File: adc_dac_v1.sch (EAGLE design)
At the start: 24 parts, among them IC2 LT6220, IC4 LT6220, U2 DAC8832IRGYR, U4 OPA353NA/3K, U7 DAC8832IRGYR, U8 OPA353NA/3K

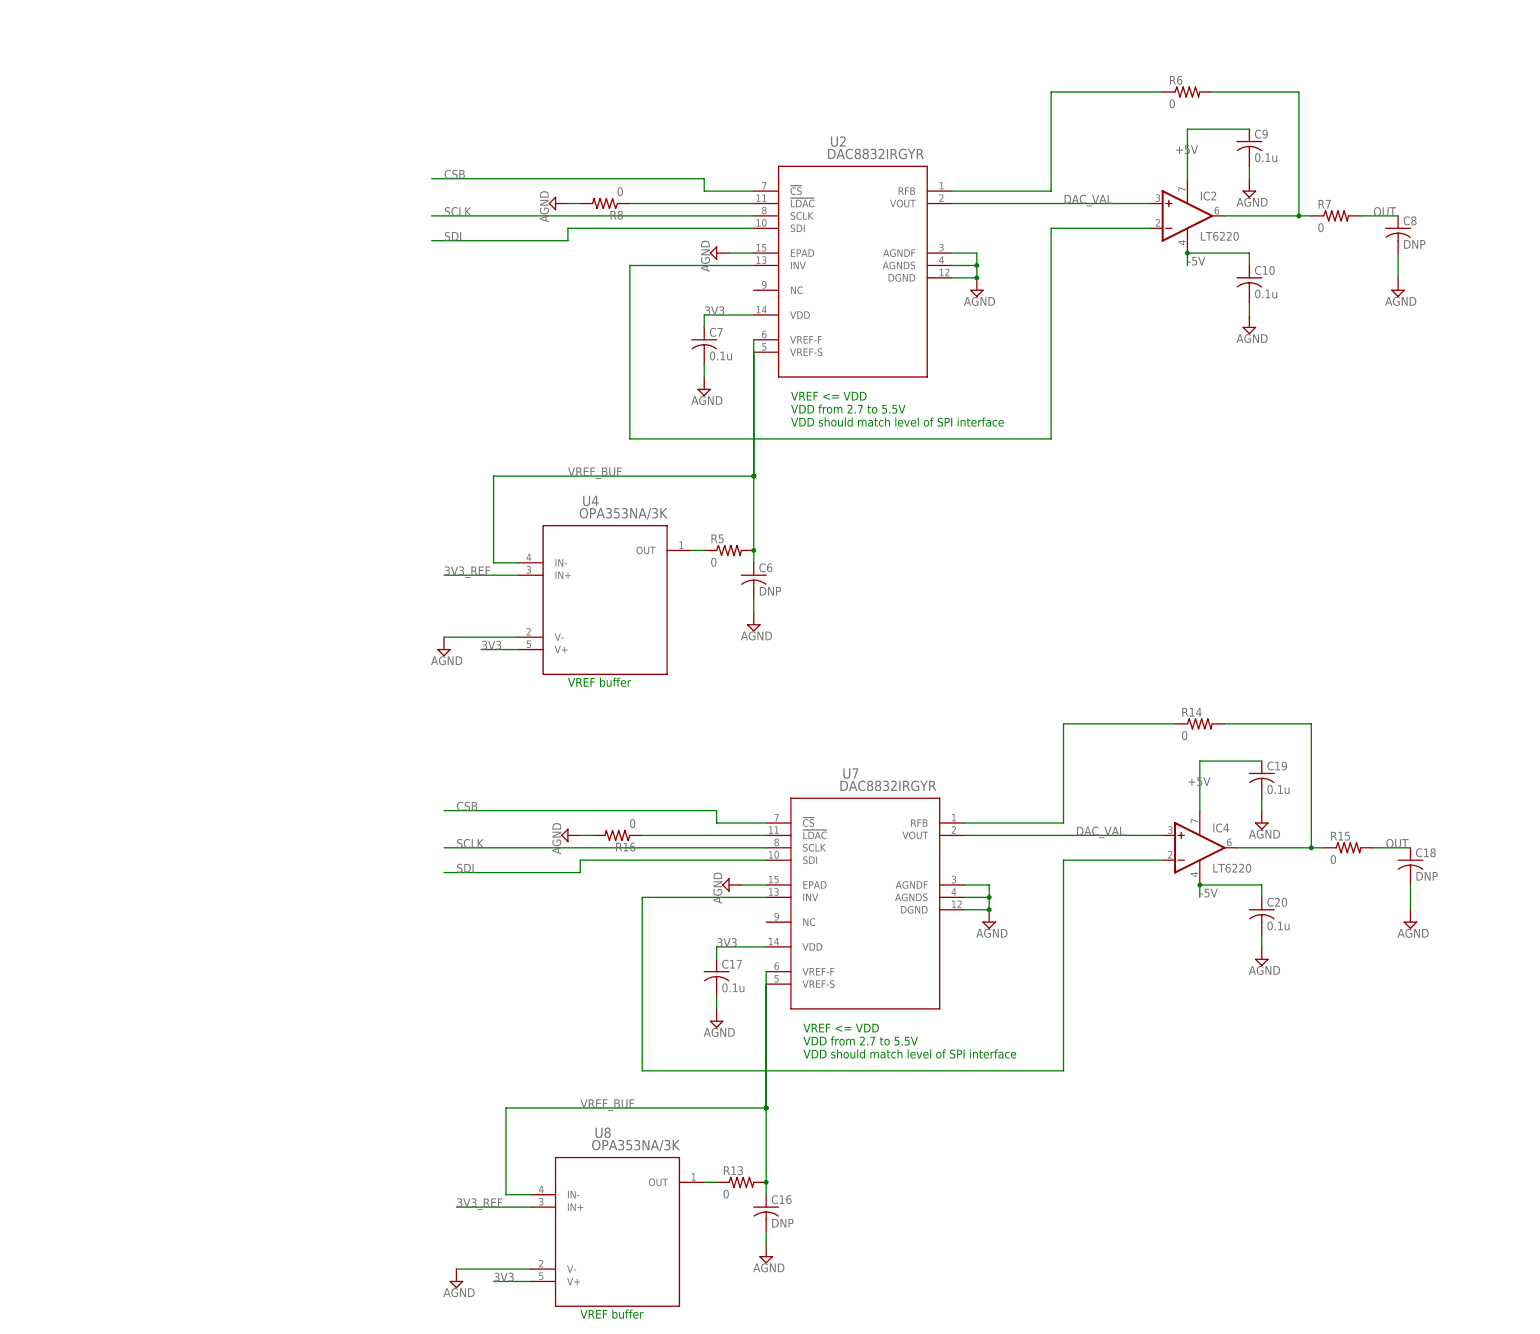
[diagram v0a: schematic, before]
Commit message: updates to DAC design
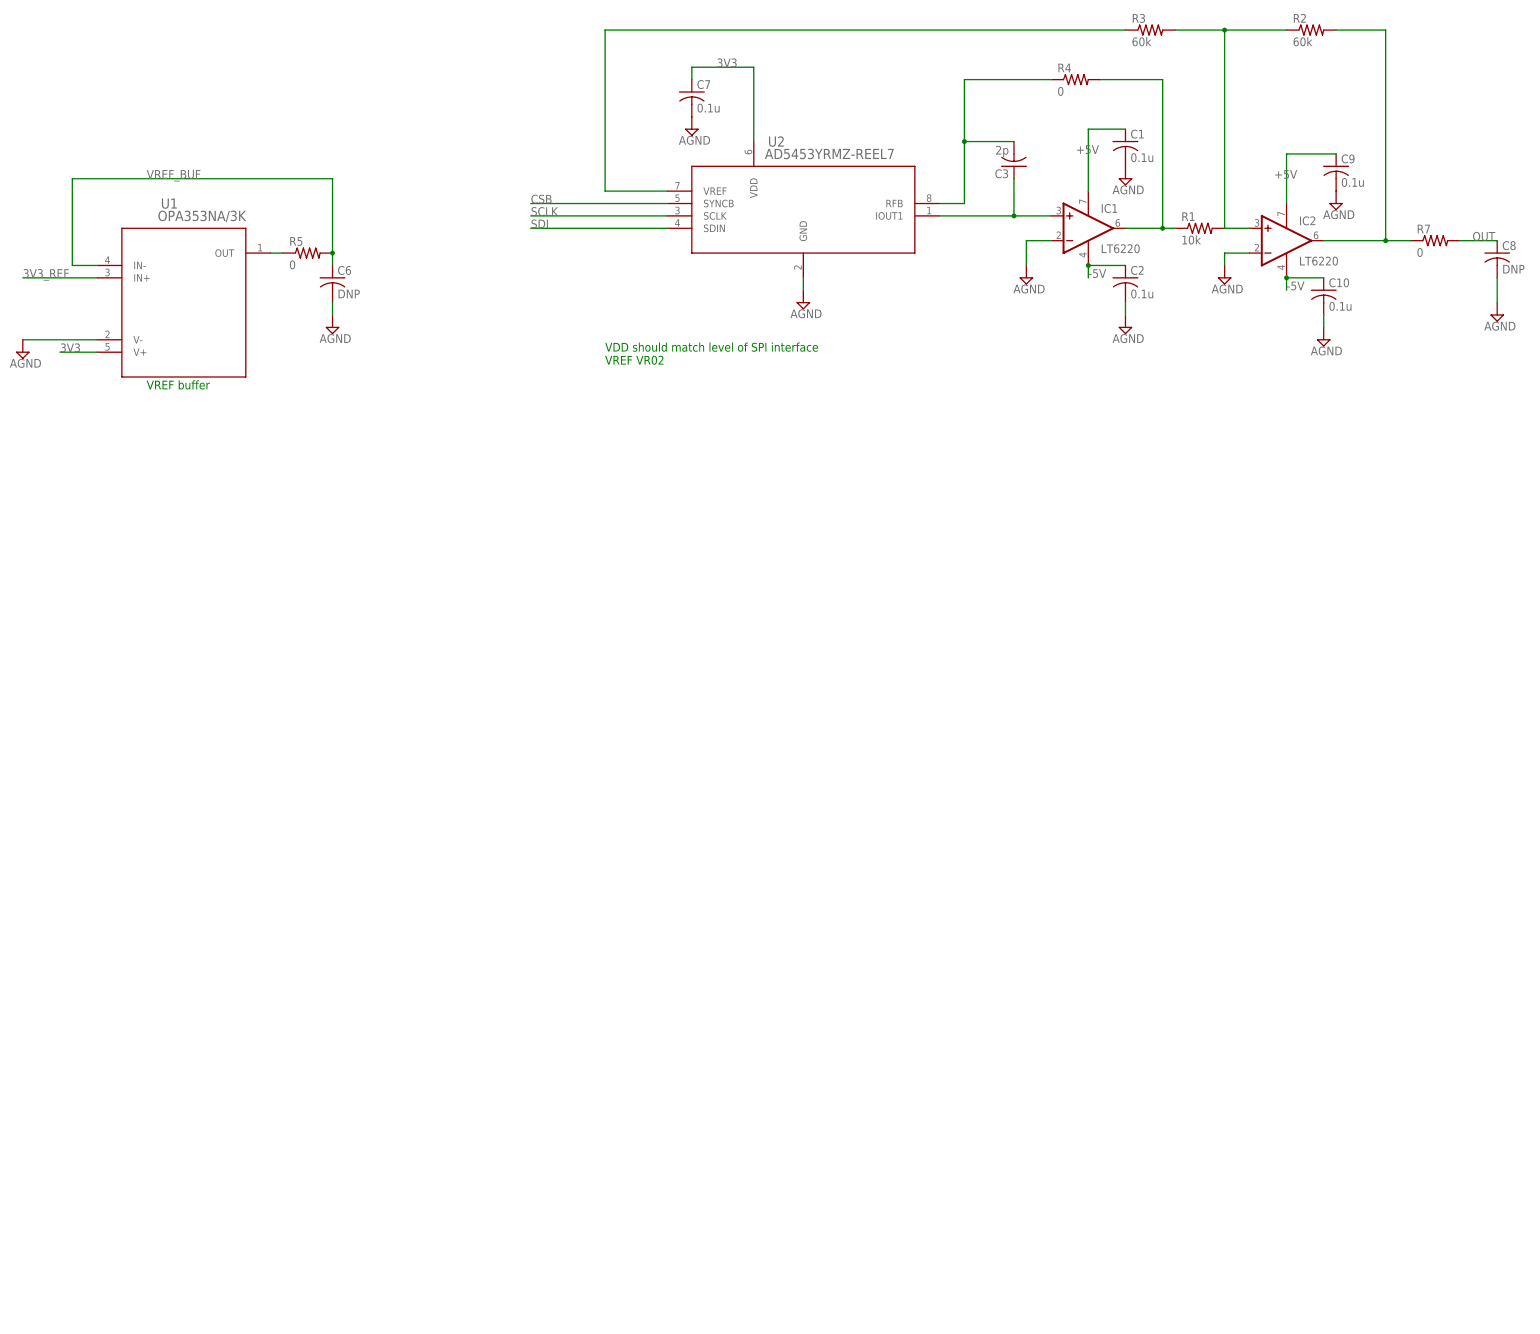
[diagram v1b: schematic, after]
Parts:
- removed C16, C18: DNP, rcl:C-USC0603
- removed C17, C19, C20: 0.1u, rcl:C-USC0603
- removed IC4: LT6220, linear:MCP601SN
- removed R13, R14, R15, R16, R6, R8: 0, rcl:R-US_R0603
- removed U4, U8: OPA353NA/3K, AD7960:OPA353NA/3K
- removed U7: DAC8832IRGYR, AD7960:DAC8832IRGYR
- added C1, C2: 0.1u, rcl:C-USC0603
- added C3: 2p, rcl:C-USC0603
- added IC1: LT6220, linear:MCP601SN
- added R1: 10k, rcl:R-US_R0603
- added R2, R3: 60k, rcl:R-US_R0603
- added R4: 0, rcl:R-US_R0603
- added U1: OPA353NA/3K, open_covg:OPA353NA/3K
- U2: value DAC8832IRGYR -> AD5453YRMZ-REEL7; device AD7960:DAC8832IRGYR -> open_covg:AD5453YRMZ-REEL7
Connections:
- removed net N$15: R14.1, U7.RFB
- removed net N$16: R16.1, U7.!LDAC
- removed net N$8: R8.1, U2.!LDAC
- new net CLK+: R2.1, U1.CLK+
- new net CLK-: R2.2, U1.CLK-
- new net CNV+: U1.CNV+
- new net CNV-: U1.CNV-
- new net D+: U1.D+
- new net D-: U1.D-
- new net DCO+: U1.DCO+
- new net DCO-: U1.DCO-
- new net DIFF_IN+: R4.1
- new net EN0: U1.EN0
- new net EN1: U1.EN1
- new net EN2: U1.EN2
- new net EN3: U1.EN3
- new net IN-: U1.IN-
- new net N$1: C3.1, IC1.+IN, IC1.IN-, IC1.OUT, R1.1, U2.IOUT1
- new net N$4: IC1.OUT, R1.1, R4.2, U1.VDD2_3
- new net REF_5V: IC1.IN+
- net +5V: now also C1.1, IC1.V+, U1.VDD1, U1.VDD1_2, U1.VDD1_3; no longer C19.1, IC4.V+
- net -5V: now also C2.1, IC1.V-; no longer C20.1, IC4.V-
- net 1.8V: now also C3.1, U1.VDD2, U1.VDD2_2, U1.VIO
- net 3V3: now also C2.1, U1.V+, U1.VDD; no longer C17.1, U4.V+, U7.VDD, U8.V+
- net 3V3_REF: now also U1.IN+; no longer U4.IN+, U8.IN+
- net AGND: now also C1.2, C2.2, C3.2, IC1.-IN, IC2.-IN, R4.1, R4.2, U1.!LDAC, U1.AGNDF, U1.AGNDS, U1.DGND, U1.EPAD, U1.V-, U2.GND; no longer C16.2, C17.2, C18.2, C19.2, C20.2, R16.2, R8.2, U2.AGNDF, U2.AGNDS, U2.DGND, U2.EPAD, U4.V-, U7.AGNDF, U7.AGNDS, U7.DGND, U7.EPAD, U8.V-
- net AMP_PWR+: now also C1.1, IC1.+VS
- net CSB: now also U1.!CS, U2.SYNCB; no longer U2.!CS, U7.!CS
- net DAC_VAL: now also IC1.+IN, U1.VOUT; no longer IC2.+IN, IC4.+IN, U2.VOUT, U7.VOUT
- net GND: now also C1.2, C2.2, C3.2, IC1.-VS, R3.1, U1.EPAD, U1.GND, U1.GND_2, U1.REFIN, U1.REF_GND, U1.REF_GND_2, U1.REF_GND_3
- net IN+: now also U1.IN+; no longer R13.2
- net N$11: no longer R6.1, R8.2
- net N$12: no longer R6.2
- net N$13: no longer IC4.-IN, IC4.OUT, R14.2, R15.1, U7.INV
- net N$14: no longer R13.1, U8.OUT
- net N$2: now also C3.2, IC1.-IN, IC1.OUT, R2.2, R3.1, R4.1, R4.2, U1.INV, U2.RFB; no longer R8.1
- net N$3: now also C2.1, IC2.+IN, R1.2, R2.1, R3.2, U1.RFB
- net N$5: now also R2.2; no longer IC2.-IN, R13.1, R6.2, U2.INV
- net N$6: now also C1.1, R1.2, U1.OUT, U1.VREF-F, U1.VREF-S; no longer U4.OUT
- net N$7: now also R3.1, U2.VREF; no longer R6.1, U2.RFB
- net OUT: now also C3.1, R3.2; no longer C18.1, R15.2
- net REF: now also R1.2, U1.REF, U1.REF_2, U1.REF_3, U1.REF_4
- net SCLK: now also U1.SCLK; no longer U7.SCLK
- net SDI: now also U1.SDI, U2.SDIN; no longer U2.SDI, U7.SDI
- net VCM: now also U1.VCM
- net VREF_BUF: now also U1.IN-; no longer C16.1, R13.2, U2.VREF-F, U2.VREF-S, U4.IN-, U7.VREF-F, U7.VREF-S, U8.IN-
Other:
- note added: "VDD should match level of SPI interface VREF VR02"
- moved on the sheet: C10, C6, C7, C8, C9, IC2, R5, R7
